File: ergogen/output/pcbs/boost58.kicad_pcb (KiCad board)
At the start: 2 copper layers, 144.3 x 128.5 mm, 104 parts, among them SW1 ${REFERENCE}, SW10 ${REFERENCE}, SW11 ${REFERENCE}, SW12 ${REFERENCE}, SW13 ${REFERENCE}, SW14 ${REFERENCE}, SW15 ${REFERENCE}, SW16 ${REFERENCE}, SW17 ${REFERENCE}, SW18 ${REFERENCE}, SW19 ${REFERENCE}, SW2 ${REFERENCE}, SW20 ${REFERENCE}, SW21 ${REFERENCE}, SW22 ${REFERENCE}, SW23 ${REFERENCE}, SW24 ${REFERENCE}, SW25 ${REFERENCE}, SW26 ${REFERENCE}, SW27 ${REFERENCE}, SW28 ${REFERENCE}, SW29 ${REFERENCE}, SW3 ${REFERENCE}, SW4 ${REFERENCE}, SW5 ${REFERENCE}, SW6 ${REFERENCE}, SW7 ${REFERENCE}, SW8 ${REFERENCE}, SW9 ${REFERENCE}

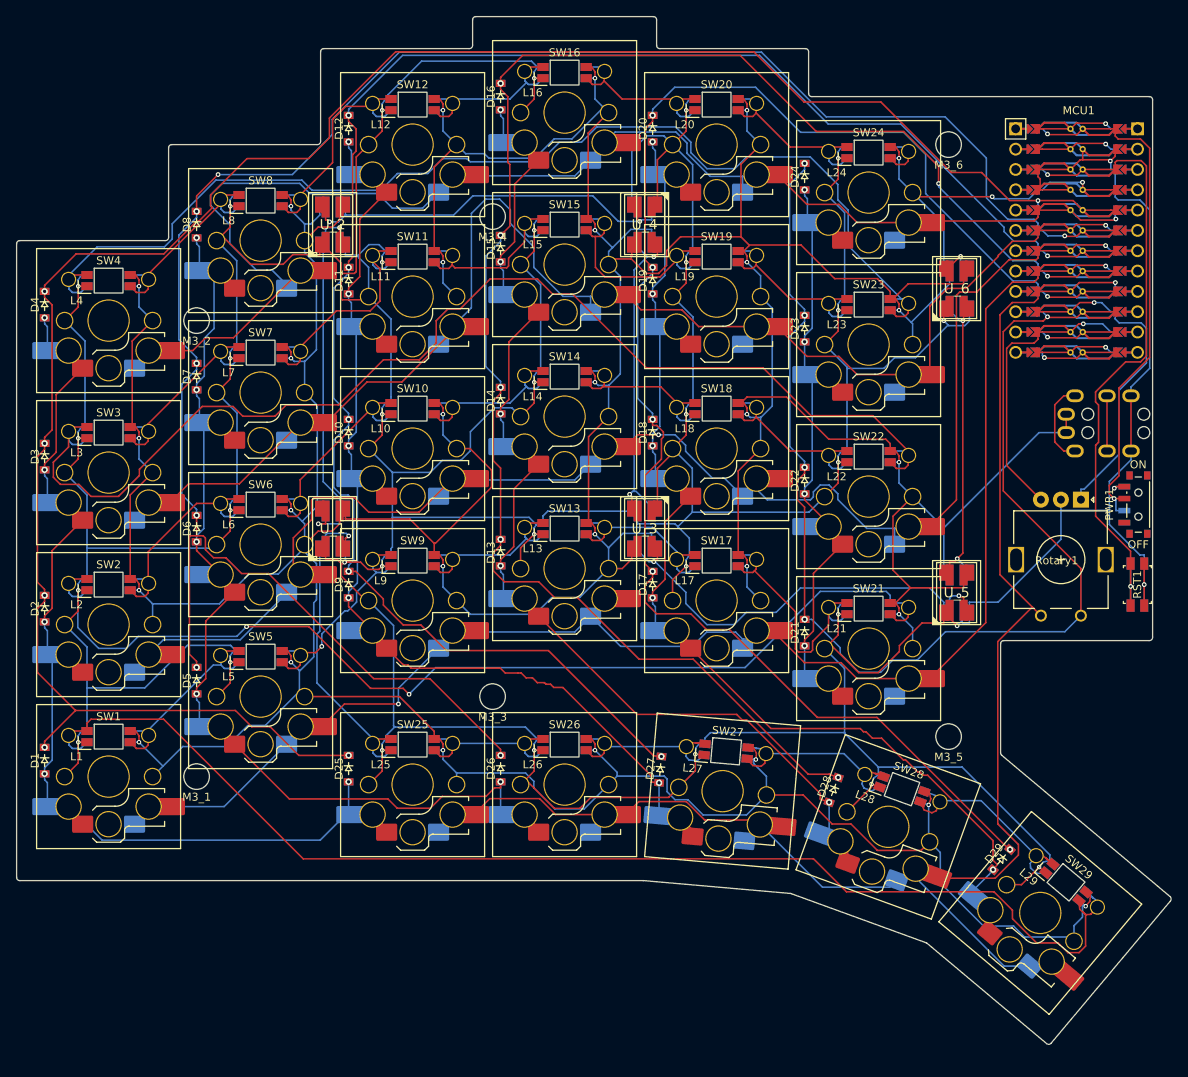
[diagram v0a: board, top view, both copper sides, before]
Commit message: re-generated circuit board and outlines, ran autotrace -- v0.2 almost ready!
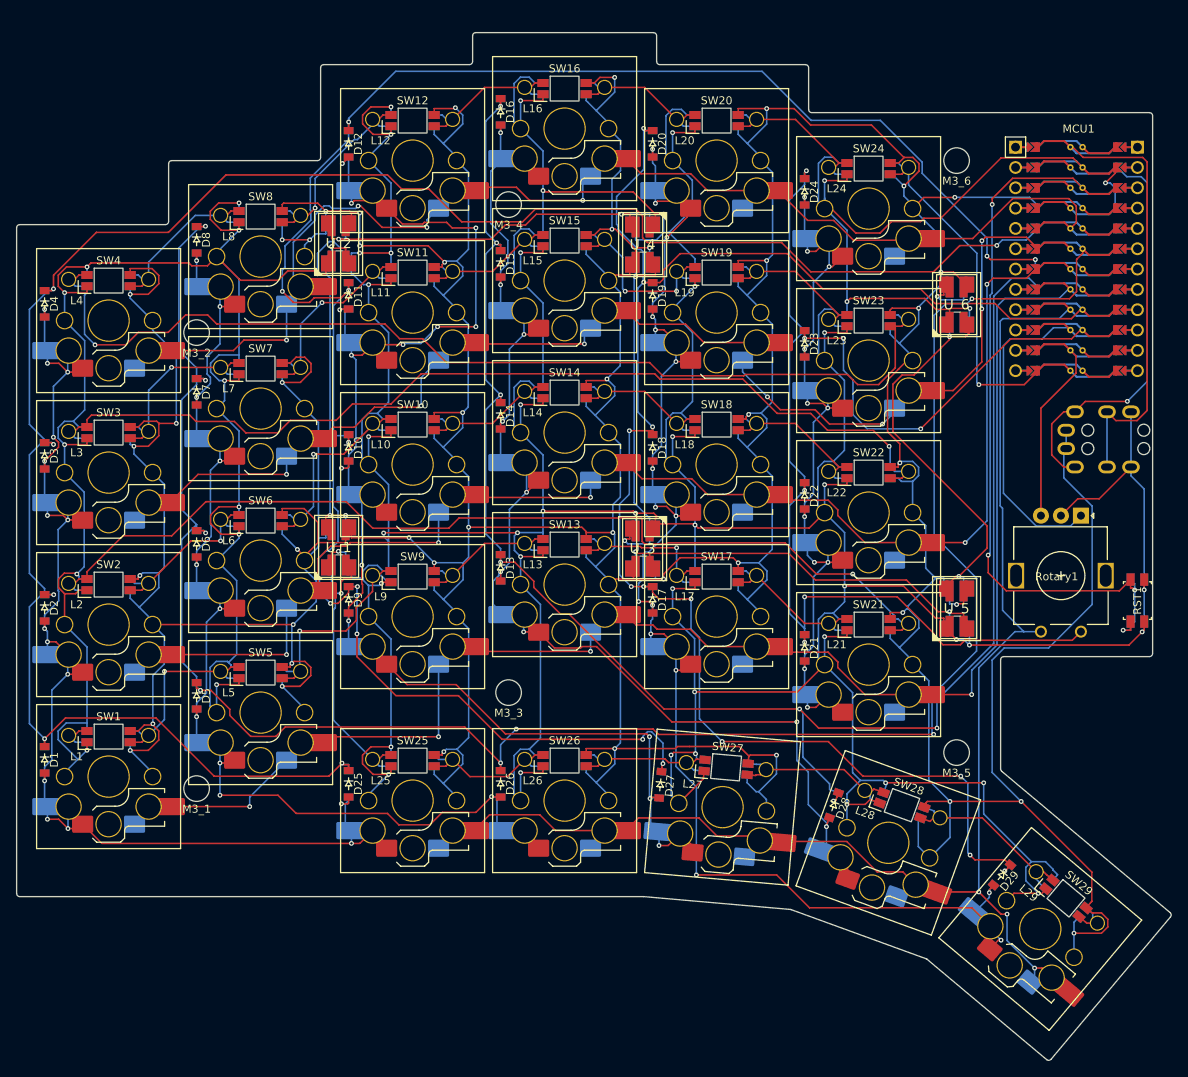
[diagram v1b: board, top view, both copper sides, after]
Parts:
- removed PWR1: , ceoloide:power_switch_smd_side
- moved U_3 2.51 mm to (106.8, 91.5)
- moved U_4 2.51 mm to (106.8, 53.5)
- moved M3_4 2.50 mm to (90.0, 48.5)
- moved U_2 2.47 mm to (68.8, 53.4)
- moved U_1 2.47 mm to (68.8, 91.3)
- moved MCU1 2.29 mm to (161.0, 55.3)
- moved M3_5 2.24 mm to (146.0, 117.0)
- moved M3_6 2.24 mm to (146.0, 43.0)
- moved M3_3 2.06 mm to (90.0, 109.5)
- moved SW28 2.00 mm to (137.5, 128.3)
- moved L10 2.00 mm to (78.0, 76.0)
- moved L11 2.00 mm to (78.0, 57.0)
- moved L12 2.00 mm to (78.0, 38.0)
- moved L13 2.00 mm to (97.0, 91.0)
- moved L14 2.00 mm to (97.0, 72.0)
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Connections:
- net LED01 renamed r0c1
- net LED02 renamed r0c2
- net LED03 renamed r0c3
- net LED04 renamed r0c4
- net LED05 renamed r0c5
- net LED11 renamed r1c1
- net LED12 renamed r1c2
- net LED13 renamed r1c3
- net LED14 renamed r1c4
- net LED15 renamed r1c5
- net LED20 renamed r2c0
- net LED21 renamed r2c1
- net LED22 renamed r2c2
- net LED23 renamed r2c3
- net LED24 renamed r2c4
- net LED25 renamed r2c5
- net LED30 renamed r3c0
- net LED31 renamed r3c1
- net LED32 renamed r3c2
- net LED33 renamed r3c3
- net LED34 renamed r3c4
- net LED35 renamed r3c5
- net LED40 renamed r4c0
- net LED41 renamed r4c1
- net LED42 renamed r4c2
- net LED43 renamed r4c3
- net LED44 renamed r4c4
- net LED45 renamed r4c5
- net LEDu01 renamed u01
- net LEDu02 renamed u02
- net LEDu03 renamed u03
- net LEDu04 renamed u04
- net LEDu05 renamed u05
- net LEDu06 renamed u06
- L1 pad 4: LED10 -> r1c0
- L24 pad 2: LED -> P9
- L29 pad 2: LED10 -> c1c0
- TRRS1 pad 2: D0 -> P0
- TRRS1 pad 3: D1 -> P1
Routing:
- net GND: track 957.5 -> 1117.7 mm, vias 34 -> 57
- net LED10: track 159.4 -> 0.00 mm
- net VCC: track 894.7 -> 1006.7 mm, vias 31 -> 45
- net RAW: track 66.2 -> 0.00 mm, vias 2 -> 0
- net P1: track 10.2 -> 54.4 mm, vias 1 -> 0
- net DP19: track 137.0 -> 180.9 mm, vias 5 -> 14
- net P0: track 10.3 -> 51.3 mm
- net P9: track 10.2 -> 44.4 mm
- net DP15: track 146.5 -> 179.1 mm, vias 5 -> 16
- net r3c0: track 152.4 -> 122.2 mm, vias 0 -> 1
- net P3: track 188.5 -> 161.9 mm, vias 1 -> 7
- net P19: track 221.9 -> 248.4 mm, vias 6 -> 11
- net P2: track 186.2 -> 161.1 mm, vias 1 -> 4
- net P4: track 198.3 -> 176.8 mm, vias 2 -> 5
- net P6: track 208.1 -> 191.0 mm, vias 1 -> 3
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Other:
- outline, holes or cut-outs redrawn
